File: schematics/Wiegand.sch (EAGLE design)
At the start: 82 parts, among them J1 AVR_SPI_PRG_6NS, U1 ATMEGA168, U2 RS485_SP491, U3 MIC5219 5V, U4 MOC3063, U5 MOC3063, U6 MOC3063, U7 MOC3063, U8 MOC3063, U9 MOC3063, X1 RJ45-8PTH, X2 RJ45-8PTH, Y1 16Mhz

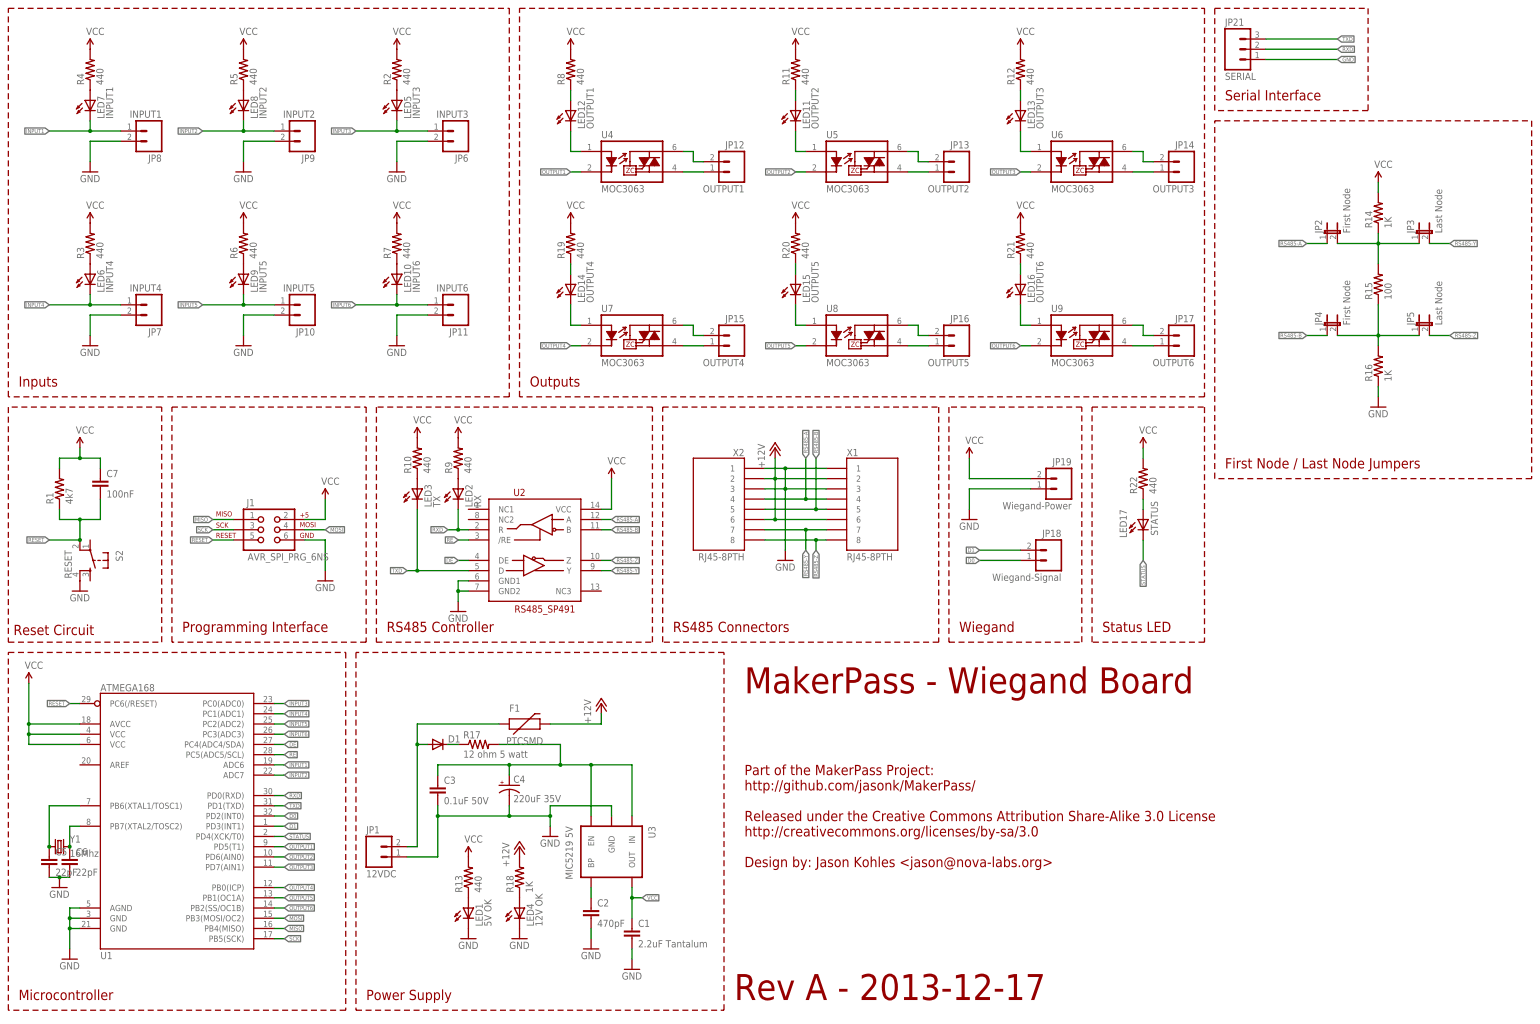
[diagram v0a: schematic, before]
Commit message: Board Rev B
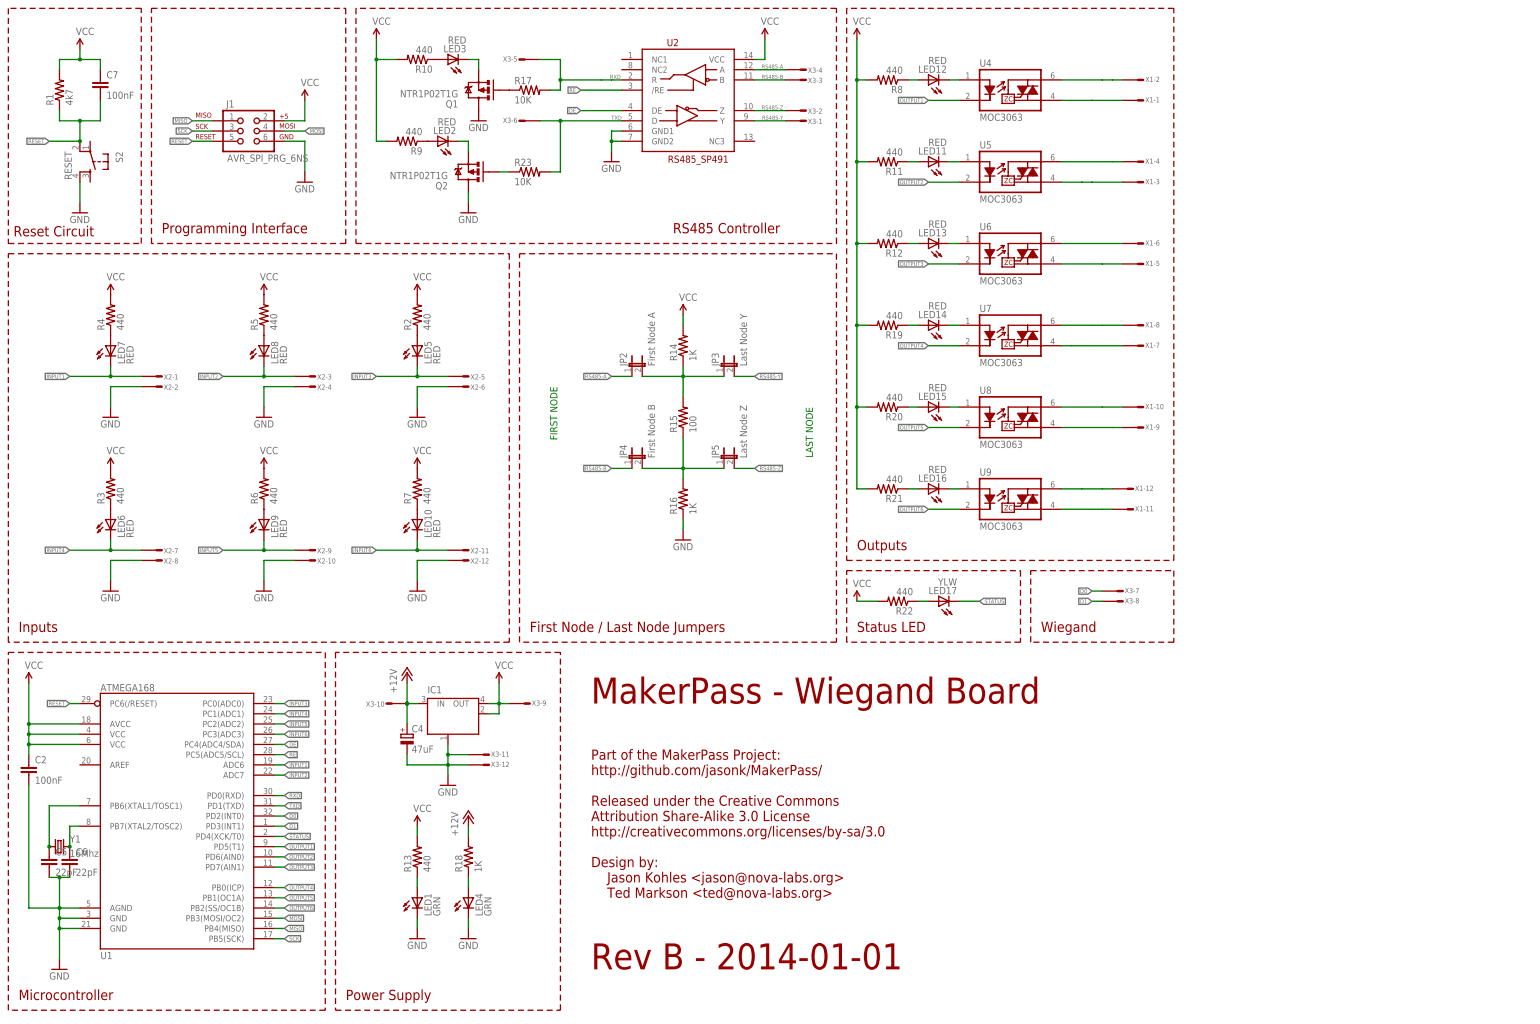
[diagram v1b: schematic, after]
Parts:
- removed C1: 2.2uF Tantalum, SparkFun-Capacitors:CAP0603-CAP
- removed C3: 0.1uF 50V, SparkFun-Capacitors:CAP0603-CAP
- removed D1: (no value), SparkFun:DIODESMA
- removed F1: PTCSMD, SparkFun:PTCSMD
- removed JP1: 12VDC, SparkFun:M025MM
- removed JP10: INPUT5, SparkFun:M023.5MM
- removed JP11: INPUT6, SparkFun:M023.5MM
- removed JP12: OUTPUT1, SparkFun:M023.5MM
- removed JP13: OUTPUT2, SparkFun:M023.5MM
- removed JP14: OUTPUT3, SparkFun:M023.5MM
- removed JP15: OUTPUT4, SparkFun:M023.5MM
- removed JP16: OUTPUT5, SparkFun:M023.5MM
- removed JP17: OUTPUT6, SparkFun:M023.5MM
- removed JP18: Wiegand-Signal, SparkFun:M023.5MM
- removed JP19: Wiegand-Power, SparkFun:M023.5MM
- removed JP21: SERIAL, SparkFun-Connectors:M03PTH
- removed JP6: INPUT3, SparkFun:M023.5MM
- removed JP7: INPUT4, SparkFun:M023.5MM
- removed JP8: INPUT1, SparkFun:M023.5MM
- removed JP9: INPUT2, SparkFun:M023.5MM
- removed U3: MIC5219 5V, SparkFun-PowerIC:V_REG_MIC52195V
- added IC1: MC33269ST-3.3T3, linear:MC33269ST-3.3T3
- added Q1, Q2: NTR1P02T1G, SparkFun:MOSFET-PCHANNELSMD
- added R23: 10K, SparkFun:RESISTOR0603-RES
- added X3: (no value), LumisenseV6:CON-1X12-TERMBLOCK-3.5MM
- C2: value 470pF -> 100nF; device SparkFun-Capacitors:CAP0603-CAP -> SparkFun:CAP0603-CAP; MFG_PN (none) -> 0603YC104KAT2A
- C4: value 220uF 35V -> 47uF; device SparkFun-Capacitors:CAP_POLD -> rcl:CPOL-EUD; MFG_PN (none) -> EMVA250ADA470MF55G
- C5, C6: MFG_PN (none) -> 06035A220JAT2A
- C7: MFG_PN (none) -> 0603YC104KAT2A
- JP2: value First Node -> First Node A; MFG_PN (none) -> 1x2 pin header
- JP3: value Last Node -> Last Node Y; MFG_PN (none) -> 1x2 pin header
- JP4: value First Node -> First Node B; MFG_PN (none) -> 1x2 pin header
- JP5: value Last Node -> Last Node Z; MFG_PN (none) -> 1x2 pin header
- LED1: value 5V OK -> GRN; MFG_PN (none) -> LG R971-KN-1
- LED10: value INPUT6 -> RED; MFG_PN (none) -> LY R976-PS-36
- LED11: value OUTPUT2 -> RED; MFG_PN (none) -> LY R976-PS-36
- LED12: value OUTPUT1 -> RED; MFG_PN (none) -> LY R976-PS-36
- LED13: value OUTPUT3 -> RED; MFG_PN (none) -> LY R976-PS-36
- LED14: value OUTPUT4 -> RED; MFG_PN (none) -> LY R976-PS-36
- LED15: value OUTPUT5 -> RED; MFG_PN (none) -> LY R976-PS-36
- LED16: value OUTPUT6 -> RED; MFG_PN (none) -> LY R976-PS-36
- LED17: value STATUS -> YLW; MFG_PN (none) -> LY R976-PS-36
- LED2: value RX -> RED; MFG_PN (none) -> LY R976-PS-36
- LED3: value TX -> RED; MFG_PN (none) -> LY R976-PS-36
- LED4: value 12V OK -> GRN; MFG_PN (none) -> LG R971-KN-1
- LED5: value INPUT3 -> RED; MFG_PN (none) -> LY R976-PS-36
- LED6: value INPUT4 -> RED; MFG_PN (none) -> LY R976-PS-36
- LED7: value INPUT1 -> RED; MFG_PN (none) -> LY R976-PS-36
- LED8: value INPUT2 -> RED; MFG_PN (none) -> LY R976-PS-36
- LED9: value INPUT5 -> RED; MFG_PN (none) -> LY R976-PS-36
- R1: MFG_PN (none) -> ERJ-3GEYJ472V
- R10, R11, R12, R13, R19, R2, R20, R21, R22, R3, R4, R5, R6, R7, R8, R9: MFG_PN (none) -> ERJ3EKF3300V
- R14, R15, R16, R18: MFG_PN (none) -> ERJ-3EKF1001V
- R17: value 12 ohm 5 watt -> 10K; MFG_PN (none) -> ERJ3EKF3300V
- S2: MFG_PN (none) -> PTS525SM10SMTRLFS
- U1: MFG_PN (none) -> ATMEGA168-20AU; OCTOPART atmega168p-20au-atmel-5825895 -> (none)
- U2: MFG_PN (none) -> SP491EEN-L
- U4, U5, U6, U7, U8, U9: MFG_PN (none) -> MOC3063M
- X1, X2: value RJ45-8PTH -> (none); device SparkFun:RJ45-8PTH -> LumisenseV6:CON-1X12-TERMBLOCK-3.5MM; MFG_PN (none) -> OSTTE120104
- Y1: MFG_PN (none) -> FOXSDLF/160-20
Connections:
- removed net 12V_IN: D1.A, F1.1, JP1.2
- new net N$42: Q2.G, R23.1
- net +12V: now also C4.+, IC1.IN, X3-10.S; no longer F1.2, X1.2, X1.6, X2.2, X2.6
- net D0: now also X3-7.S; no longer JP18.1
- net D1: now also X3-8.S; no longer JP18.2
- net GND: now also IC1.GND/ADJ, Q1.D, Q2.D, X2-10.S, X2-12.S, X2-2.S, X2-4.S, X2-6.S, X2-8.S, X3-11.S, X3-12.S; no longer C1.2, C3.2, JP1.1, JP10.2, JP11.2, JP19.1, JP21.1, JP6.2, JP7.2, JP8.2, JP9.2, U3.GND, X1.1, X1.3, X2.1, X2.3
- net INPUT1: now also X2-1.S; no longer JP8.1
- net INPUT2: now also X2-3.S; no longer JP9.1
- net INPUT3: now also X2-5.S; no longer JP6.1
- net INPUT4: now also X2-7.S; no longer JP7.1
- net INPUT5: now also X2-9.S; no longer JP10.1
- net INPUT6: now also X2-11.S; no longer JP11.1
- net N$17: now also X1-1.S; no longer JP12.1
- net N$18: now also X1-2.S; no longer JP12.2
- net N$19: now also X1-3.S; no longer JP13.1
- net N$20: now also X1-4.S; no longer JP13.2
- net N$23: now also X1-5.S; no longer JP14.1
- net N$24: now also X1-6.S; no longer JP14.2
- net N$29: now also X1-7.S; no longer JP15.1
- net N$3: now also U8.T2, X1-9.S; no longer C2.1, U3.BP
- net N$30: now also X1-8.S; no longer JP15.2
- net N$33: now also LED2.C, Q2.S; no longer JP16.1, U8.T2
- net N$34: now also Q1.G, R17.1; no longer JP16.2, U8.T1
- net N$37: now also X1-11.S; no longer JP17.1
- net N$38: now also X1-12.S; no longer JP17.2
- net N$4: now also U8.T1, X1-10.S; no longer C3.1, C4.+, R17.2, U3.EN, U3.IN
- net N$9: now also LED3.C, Q1.S; no longer D1.C, R17.1
- net RS485-A: now also X3-4.S; no longer X1.4, X2.4
- net RS485-B: now also X3-3.S; no longer X1.5, X2.5
- net RS485-Y: now also X3-1.S; no longer X1.7, X2.7
- net RS485-Z: now also X3-2.S; no longer X1.8, X2.8
- net RXD: now also R17.2, X3-5.S; no longer JP21.2, LED2.C
- net TXD: now also R23.2, X3-6.S; no longer JP21.3, LED3.C
- net VCC: now also C2.1, IC1.OUT, IC1.OUT@1, X3-9.S; no longer C1.1, JP19.2, U3.OUT
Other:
- note added: "FIRST NODE"
- note added: "LAST NODE"
- note added: "Part of the MakerPass Project: http://github.com/jasonk/MakerPass/ Released under the Creative Commons Attribution Share-Alike 3.0 License http://creativecommons.org/licenses/by-sa/3.0 Design by: Jason Kohles <jason@nova-labs.org> Ted Markson <ted@nova-labs.org>"
- note added: "Rev B - 2014-01-01"
- note removed: "Part of the MakerPass Project: http://github.com/jasonk/MakerPass/ Released under the Creative Commons Attribution Share-Alike 3.0 License http://creativecommons.org/licenses/by-sa/3.0 Design by: Jason Kohles <jason@nova-labs.org>"
- note removed: "RS485 Connectors"
- note removed: "Rev A - 2013-12-17"
- note removed: "Serial Interface"
- moved on the sheet: C2, C4, C7, J1, JP2, JP3, JP4, JP5, LED1, LED10, LED11, LED12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
